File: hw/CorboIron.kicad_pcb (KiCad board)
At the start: 2 copper layers, 158.8 x 99.1 mm, 82 parts, among them P1 CONN_01X03, P10 CONN_01X04, P11 CONN_01X04, P2 CONN_01X03, P3 CONN_01X03, P4 Arduino_nano, P5 CONN_01X03, P6 CONN_01X04, P7 CONN_01X02, P8 CONN_01X03, P9 CONN_01X03, Q1 IPS6041RPBF, Q2 IPS6041RPBF, Q3 IPS6041RPBF, Q4 IPS6041RPBF, U1 74LS08, U10 LM741, U11 LM741, U12 LM741, U13 LM741, U14 7805, U2 LM741, U3 LM741, U4 LM741, U5 LM741, U6 LM741, U7 LM741, U8 LM741, U9 LM741

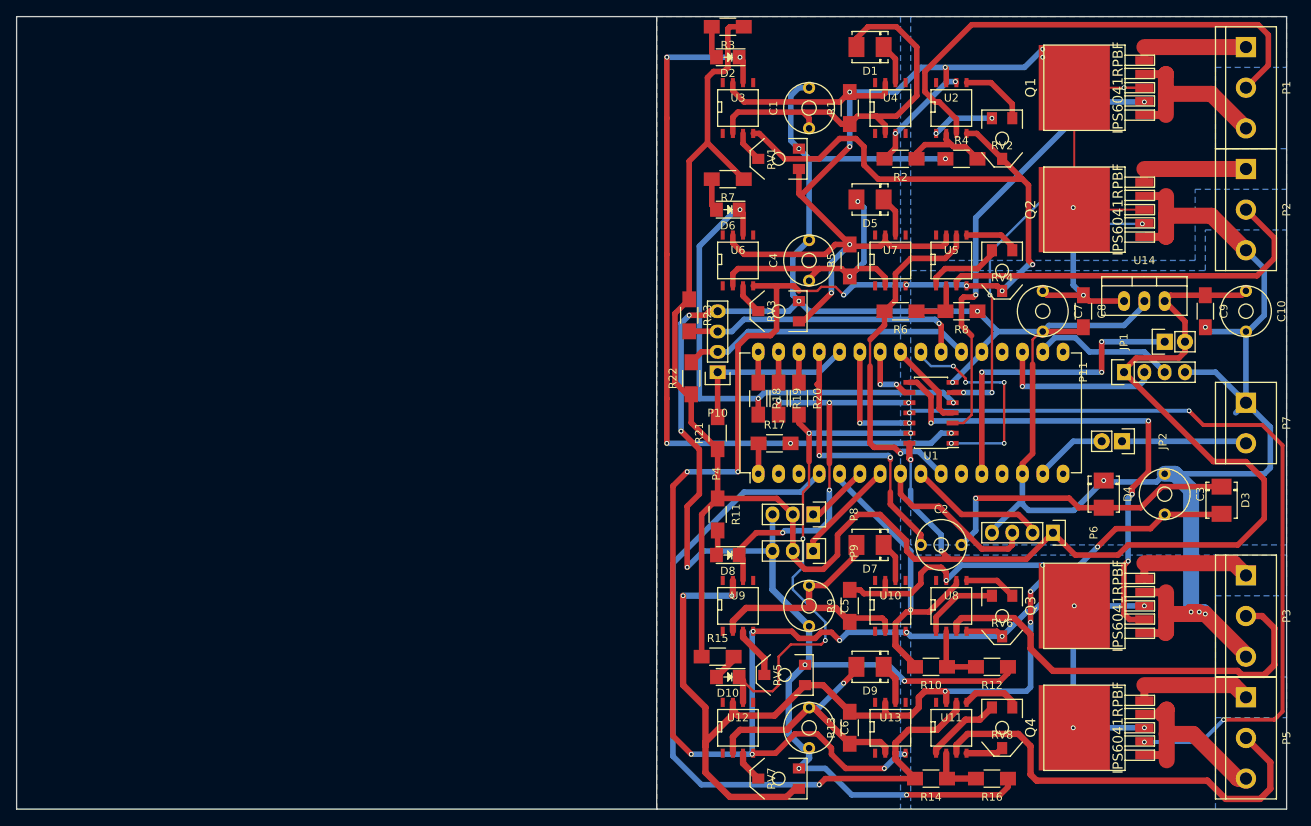
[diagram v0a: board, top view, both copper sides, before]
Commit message: Started pretty version
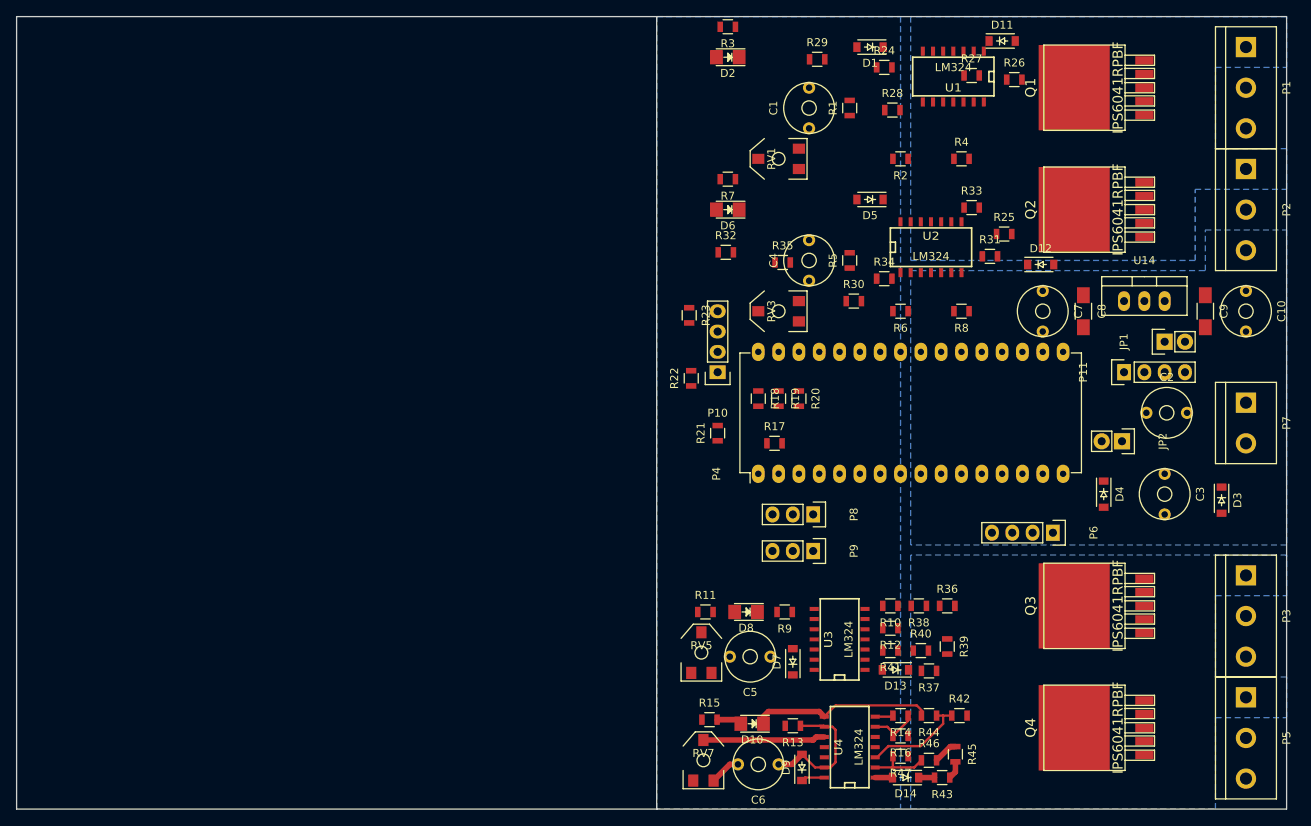
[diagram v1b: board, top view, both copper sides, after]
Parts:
- removed RV2, RV4, RV6, RV8: POT, SMD_Packages:POT_SMD
- removed U10, U11, U12, U13, U5, U6, U7, U8, U9: LM741, SMD_Packages:SOIC-8-N
- added D11: D, Diodes_SMD:SOD-123, F.Cu at (160.0, 67.8)
- added D12: D, Diodes_SMD:SOD-123, F.Cu at (164.8, 95.8)
- added D13: D, Diodes_SMD:SOD-123, F.Cu at (146.7, 146.4)
- added D14: D, Diodes_SMD:SOD-123, F.Cu at (148.0, 159.9)
- added R24: R, Resistors_SMD:R_0805, F.Cu at (145.3, 71.1)
- added R25: R, Resistors_SMD:R_0805, F.Cu at (160.3, 91.9)
- added R26: R, Resistors_SMD:R_0805, F.Cu at (161.5, 72.6)
- added R27: R, Resistors_SMD:R_0805, F.Cu at (156.2, 72.1)
- added R28: R, Resistors_SMD:R_0805, F.Cu at (146.3, 76.5)
- added R29: R, Resistors_SMD:R_0805, F.Cu at (136.9, 70.1)
- added R30: R, Resistors_SMD:R_0805, F.Cu at (141.5, 100.3)
- added R31: R, Resistors_SMD:R_0805, F.Cu at (158.5, 94.7)
- added R32: R, Resistors_SMD:R_0805, F.Cu at (125.5, 94.2)
- added R33: R, Resistors_SMD:R_0805, F.Cu at (156.2, 88.6)
- added R34: R, Resistors_SMD:R_0805, F.Cu at (145.3, 97.5)
- added R35: R, Resistors_SMD:R_0805, F.Cu at (132.6, 95.5)
- added R36: R, Resistors_SMD:R_0805, F.Cu at (153.2, 138.4)
- added R37: R, Resistors_SMD:R_0805, F.Cu at (150.9, 146.6)
- added R38: R, Resistors_SMD:R_0805, F.Cu at (149.6, 138.4)
- added R39: R, Resistors_SMD:R_0805, F.Cu at (153.2, 143.5)
- added R40: R, Resistors_SMD:R_0805, F.Cu at (149.9, 144.0)
- added R41: R, Resistors_SMD:R_0805, F.Cu at (146.1, 144.0)
- added R42: R, Resistors_SMD:R_0805, F.Cu at (154.7, 152.1)
- added R43: R, Resistors_SMD:R_0805, F.Cu at (152.5, 159.9)
- added R44: R, Resistors_SMD:R_0805, F.Cu at (150.9, 152.1)
- added R45: R, Resistors_SMD:R_0805, F.Cu at (154.2, 157.0)
- added R46: R, Resistors_SMD:R_0805, F.Cu at (150.9, 157.7)
- added R47: R, Resistors_SMD:R_0805, F.Cu at (147.3, 157.2)
- D1, D3, D4, D5, D7, D9: footprint Diodes_SMD:DO-214BA -> Diodes_SMD:SOD-123
- R1, R10, R11, R12, R13, R14, R15, R16, R17, R18, R19, R2, R20, R21, R22, R23, R3, R4, R5, R6, R7, R8, R9: footprint Resistors_SMD:R_1206_HandSoldering -> Resistors_SMD:R_0805
- U1: value 74LS08 -> LM324; footprint Housings_SOIC:SOIC-14_3.9x8.7mm_Pitch1.27mm -> SMD_Packages:SO14N
- U2, U3, U4: value LM741 -> LM324; footprint SMD_Packages:SOIC-8-N -> SMD_Packages:SO14N
- moved U4 80.1 mm to (140.8, 156.1), turned to 90 degrees
- moved U3 67.6 mm to (139.6, 142.6), turned to 90 degrees
- moved U1 42.0 mm to (153.9, 72.4)
- moved C2 32.7 mm to (180.6, 114.3)
- moved D7 17.5 mm to (133.9, 145.4), turned to 90 degrees
- moved U2 17.5 mm to (151.1, 93.5)
- moved D9 15.2 mm to (135.0, 158.6), turned to 90 degrees
- moved R12 13.6 mm to (146.1, 141.2)
- moved R16 12.6 mm to (147.3, 154.7)
- moved R11 12.3 mm to (122.9, 139.2), turned to 0 degrees
- moved RV5 10.8 mm to (122.4, 144.3), turned to 0 degrees
- moved C5 9.73 mm to (128.5, 144.8), turned to 0 degrees
- moved RV7 9.67 mm to (122.7, 157.7), turned to 0 degrees
- moved R10 9.16 mm to (146.1, 138.4)
- moved R14 8.75 mm to (147.3, 152.1)
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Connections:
- Q1 pad 2: /HTR3_CTL -> Net-(Q1-Pad2)
- Q2 pad 2: /HTR2_CTL -> Net-(Q2-Pad2)
- Q3 pad 2: /HTR1_CTL -> Net-(Q3-Pad2)
- Q4 pad 2: /HTR0_CTL' -> Net-(Q4-Pad2)
- U1 pad 1: /HTR3_EN -> /HTR3_CTL
- U1 pad 10: /TEMP1_OK -> Net-(RV1-Pad2)
- U1 pad 11: /HTR0_CTL' -> /V_NEG
- U1 pad 12: /HTR0_EN -> /TEMP3_AMP
- U1 pad 13: /TEMP0_OK -> /TEMP3_MIN
- U1 pad 14: +5V -> Net-(D1-Pad1)
- U1 pad 2: /TEMP3_OK -> Net-(R28-Pad1)
- U1 pad 3: /HTR3_CTL -> Net-(R24-Pad1)
- U1 pad 4: /HTR2_EN -> +12V
- U1 pad 5: /TEMP2_OK -> /TEMP3
- U1 pad 6: /HTR2_CTL -> Net-(R2-Pad1)
- U1 pad 7: GND -> /TEMP3_AMP
- U1 pad 8: /HTR1_CTL -> /TEMP3_OK
- U1 pad 9: /HTR1_EN -> /TEMP3_MIN
- U2 pad 1: Net-(RV2-Pad3) -> /HTR2_CTL
- U2 pad 2: Net-(R2-Pad1) -> Net-(R34-Pad1)
- U2 pad 3: /TEMP3 -> Net-(R30-Pad1)
- U2 pad 4: /V_NEG -> +12V
- U2 pad 5: Net-(RV2-Pad1) -> /TEMP2
- U2 pad 6: /TEMP3_AMP -> Net-(R6-Pad1)
- U2 pad 7: +12V -> /TEMP2_AMP
- U2 pad 8: (no net) -> /TEMP2_OK
- U3 pad 1: (no net) -> /HTR1_CTL
- U3 pad 2: /TEMP3_MIN -> Net-(R40-Pad1)
- U3 pad 3: Net-(RV1-Pad2) -> Net-(R36-Pad1)
- U3 pad 4: /V_NEG -> +12V
- U3 pad 5: (no net) -> /TEMP1
- U3 pad 6: /TEMP3_OK -> Net-(R10-Pad1)
- U3 pad 7: +12V -> /TEMP1_AMP
- U3 pad 8: (no net) -> /TEMP1_OK
- U4 pad 1: (no net) -> /HTR0_CTL'
- U4 pad 2: /TEMP3_MIN -> Net-(R46-Pad1)
- U4 pad 3: /TEMP3_AMP -> Net-(R42-Pad1)
- U4 pad 4: /V_NEG -> +12V
- U4 pad 5: (no net) -> /TEMP0
- U4 pad 6: Net-(D1-Pad1) -> Net-(R14-Pad1)
- U4 pad 7: +12V -> /TEMP0_AMP
- U4 pad 8: (no net) -> /TEMP0_OK
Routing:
- net GND: track 490.2 -> 6.95 mm, vias 17 -> 0
- net +12V: track 397.8 -> 0.00 mm, vias 21 -> 0
- net /V_NEG: track 286.2 -> 0.00 mm, vias 16 -> 0
- net +5V: track 253.2 -> 0.00 mm, vias 2 -> 0
- net /HTR0_CTL': track 100.7 -> 2.17 mm, vias 4 -> 0
- net /TEMP3_OK: track 97.1 -> 0.00 mm, vias 5 -> 0
- net /TEMP0_AMP: track 94.9 -> 2.28 mm, vias 1 -> 0
- net /TEMP2_OK: track 64.2 -> 0.00 mm, vias 3 -> 0
- net /TEMP3: track 63.3 -> 0.00 mm
- net /HTR1_CTL: track 62.2 -> 0.00 mm, vias 4 -> 0
- net /HTR3_CTL: track 56.6 -> 0.00 mm, vias 2 -> 0
- net /TEMP0: track 54.4 -> 0.00 mm
- net /TEMP1: track 54.3 -> 0.00 mm
- net /TEMP2: track 49.1 -> 0.00 mm
- net /TEMP1_OK: track 49.1 -> 0.00 mm, vias 5 -> 0
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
